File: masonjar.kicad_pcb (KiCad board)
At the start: 2 copper layers, 63.8 x 100 mm, 189 parts, among them U1 ESP32-WROOM-32

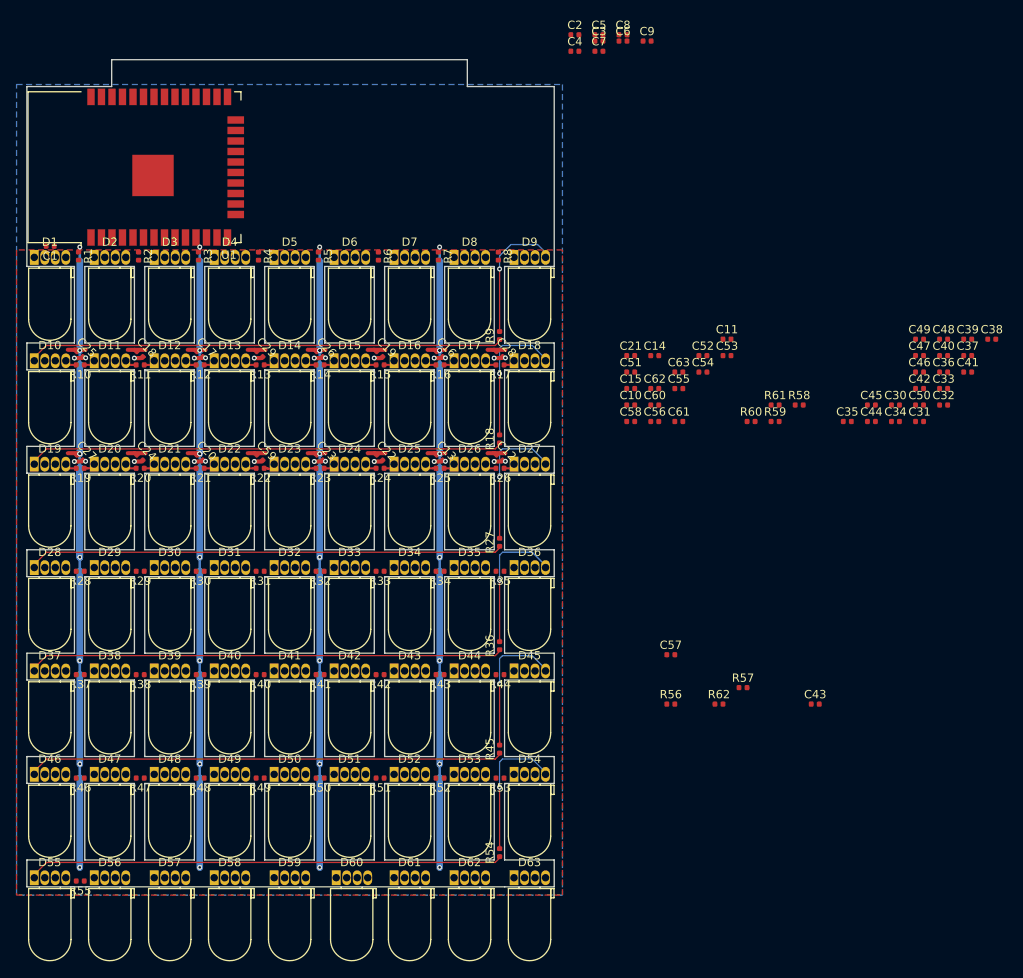
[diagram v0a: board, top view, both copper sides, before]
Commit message: working on layout
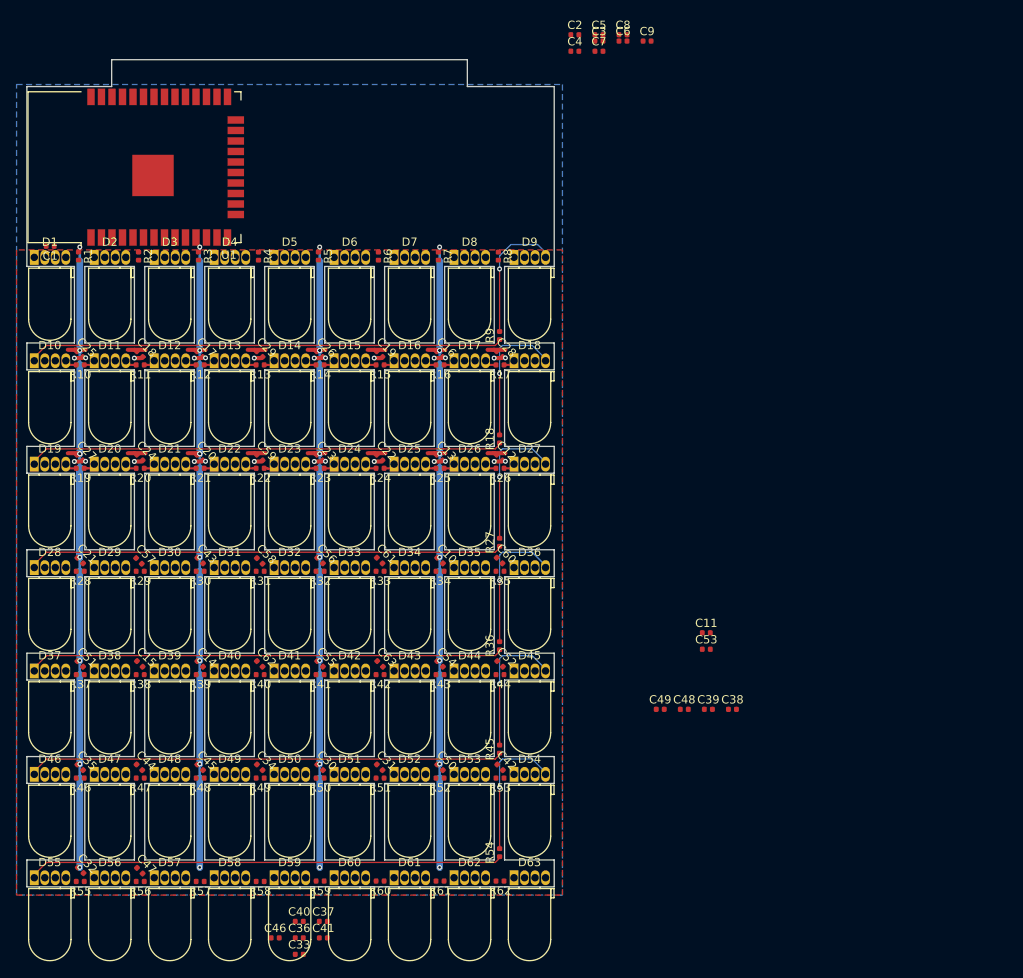
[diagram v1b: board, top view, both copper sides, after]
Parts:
- moved C32 118.5 mm to (-25.2, 98.0), turned to 315 degrees
- moved C47 113.0 mm to (-18.1, 98.0), turned to 315 degrees
- moved C46 103.7 mm to (-1.73, 106.2)
- moved C33 103.7 mm to (1.18, 108.2)
- moved C36 103.7 mm to (1.18, 106.2)
- moved C37 103.7 mm to (4.09, 104.2)
- moved C40 103.7 mm to (1.18, 104.2)
- moved C41 103.7 mm to (4.09, 106.2)
- moved C35 101.7 mm to (-25.3, 85.5), turned to 315 degrees
- moved C44 97.9 mm to (-18.1, 85.5), turned to 315 degrees
- moved C45 92.2 mm to (-10.8, 85.5), turned to 315 degrees
- moved C34 87.5 mm to (-3.60, 85.5), turned to 315 degrees
- moved R58 87.0 mm to (-3.55, 99.3), turned to 180 degrees
- moved C30 82.2 mm to (3.70, 85.5), turned to 315 degrees
- moved R59 78.2 mm to (3.70, 99.3), turned to 180 degrees
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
